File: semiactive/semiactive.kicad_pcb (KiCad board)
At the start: 2 copper layers, 85 x 85 mm, 12 parts, among them J1 5223004-2, U1 Teensy4.1

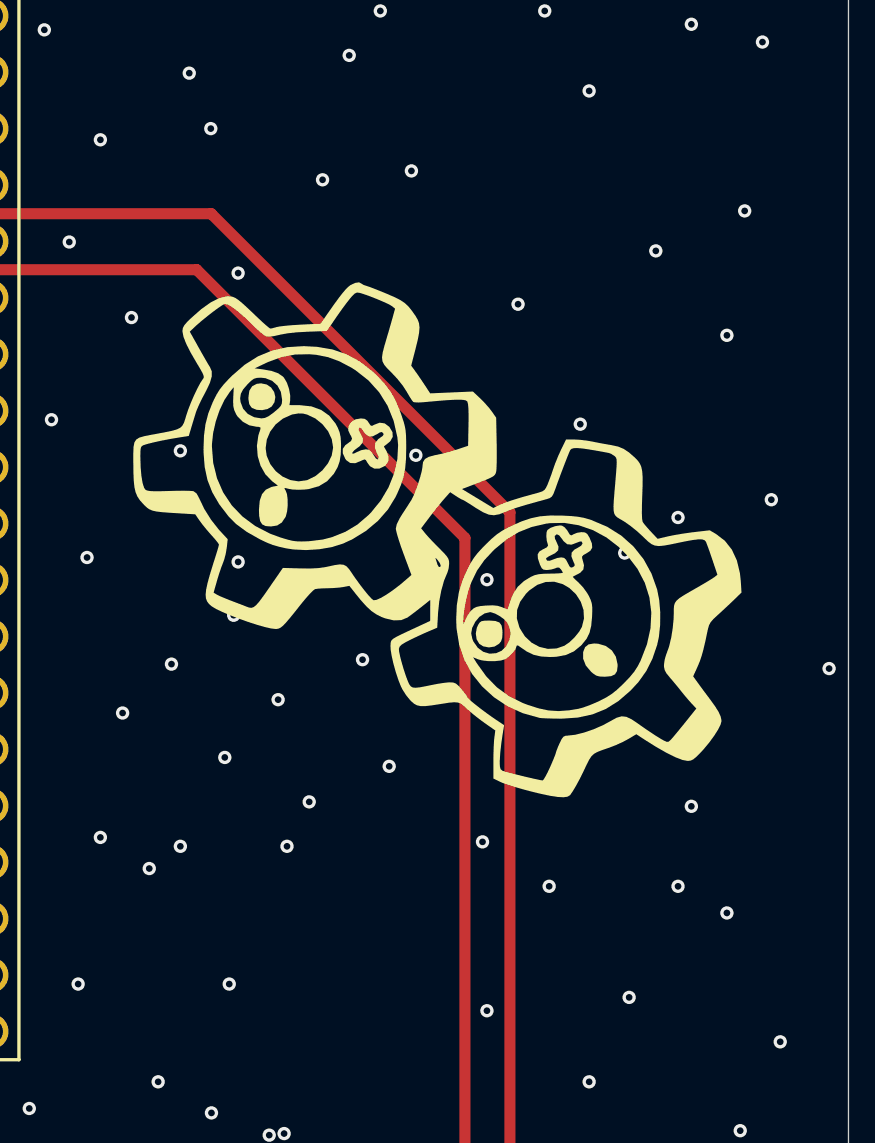
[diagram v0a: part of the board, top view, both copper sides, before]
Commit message: Update semiactive ponkerman
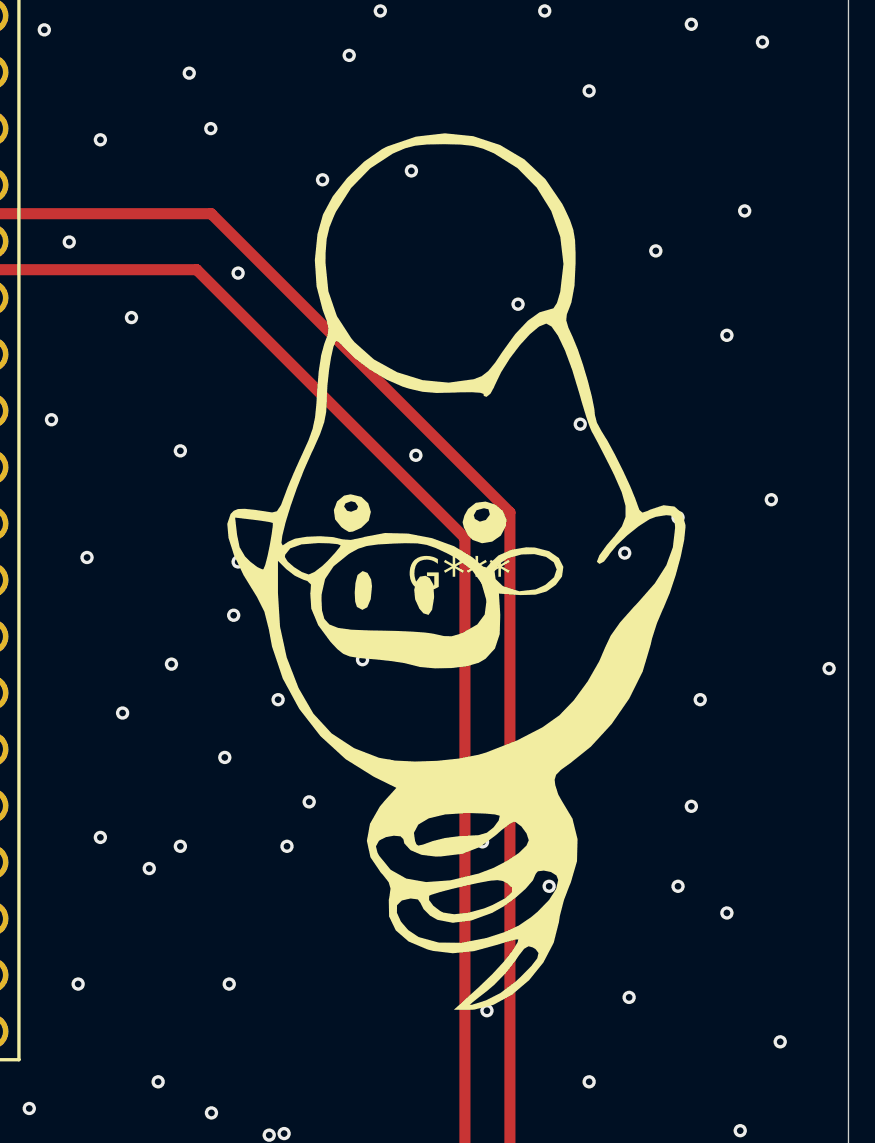
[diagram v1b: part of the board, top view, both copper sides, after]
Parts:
- moved G*** 1.83 mm to (182.1, 82.3)
